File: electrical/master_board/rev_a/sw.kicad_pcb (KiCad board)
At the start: 2 copper layers, 64.7 x 45 mm, 0 parts

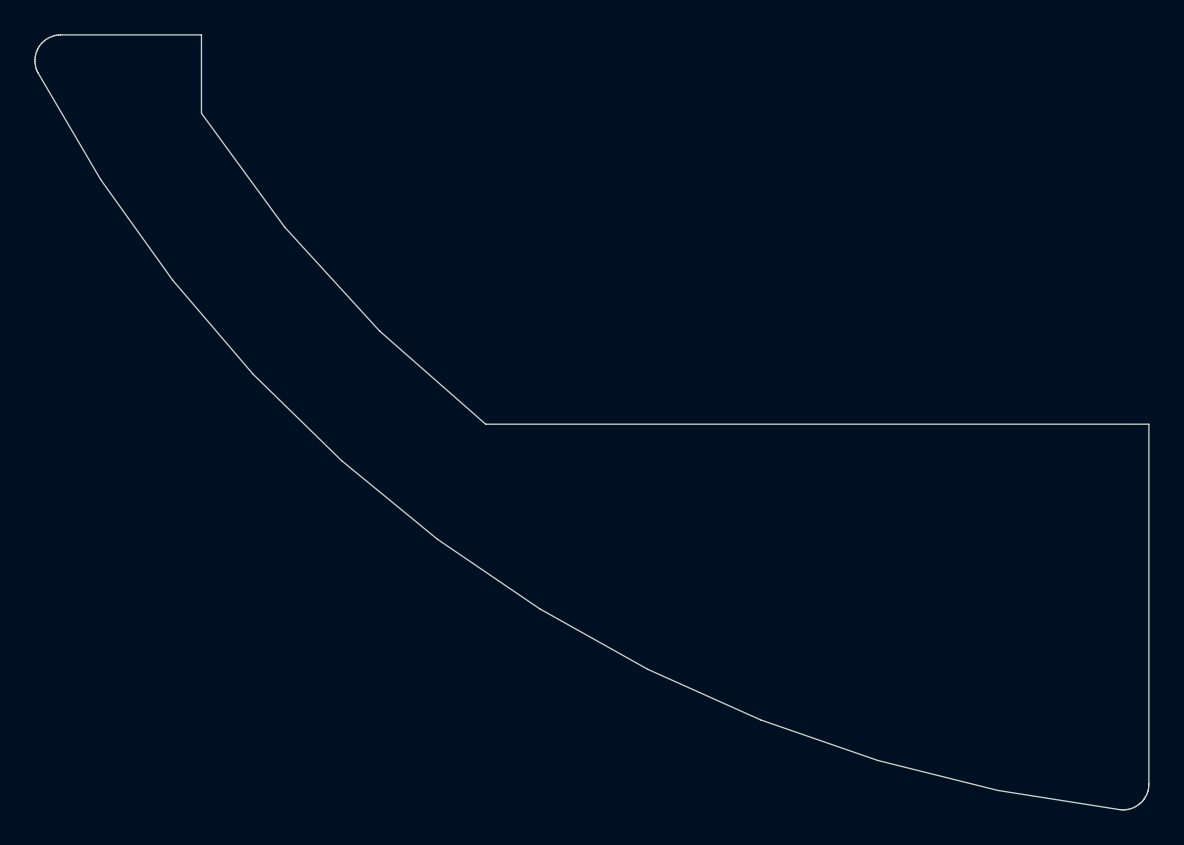
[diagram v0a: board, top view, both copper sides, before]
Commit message: Finally have everything fitting together.
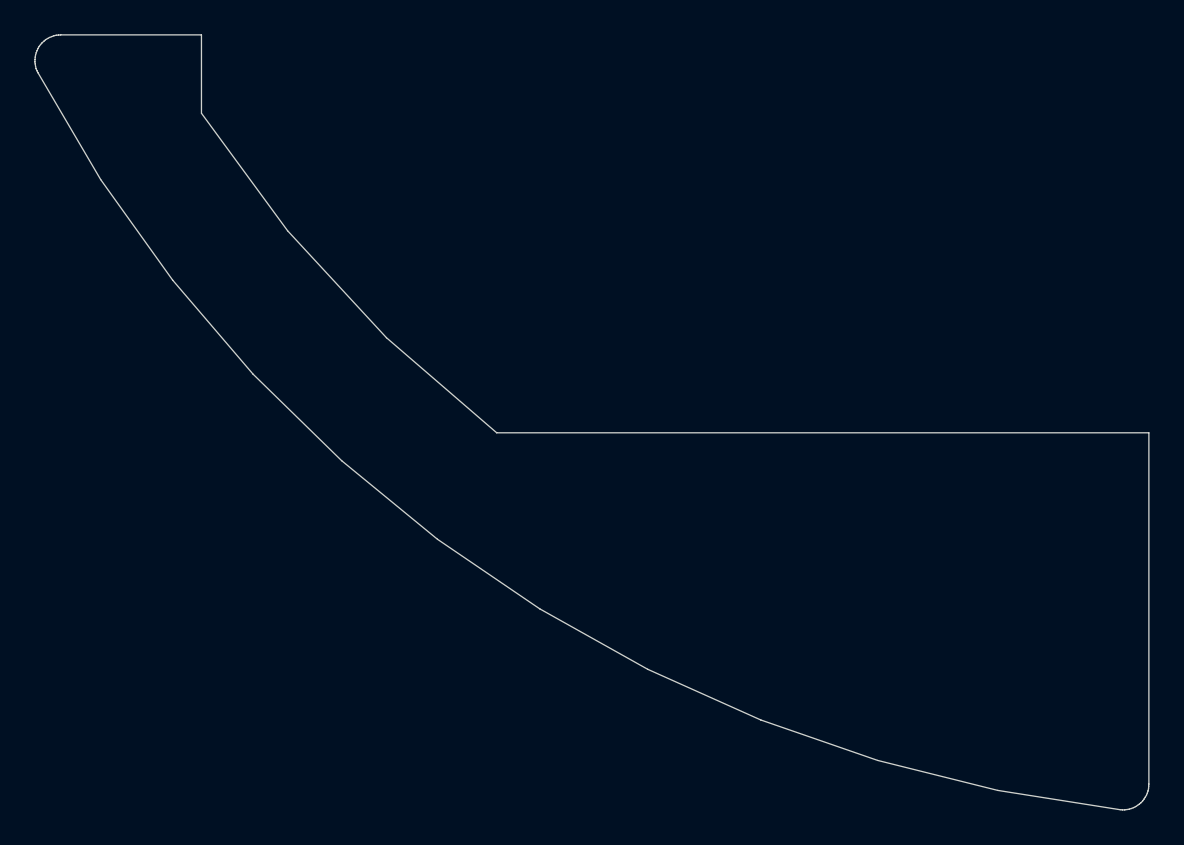
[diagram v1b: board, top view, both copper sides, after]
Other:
- outline, holes or cut-outs redrawn
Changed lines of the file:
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@@
   (gr_line (start 92.48 179.76) (end 92.49 179.62) (layer Edge.Cuts) (width 0.05))
   (gr_line (start 92.49 179.62) (end 92.5 179.49) (layer Edge.Cuts) (width 0.05))
-  (gr_line (start 92.5 179.49) (end 92.5 158.6) (layer Edge.Cuts) (width 0.05))
-  (gr_line (start 92.5 158.6) (end 54 158.6) (layer Edge.Cuts) (width 0.05))
-  (gr_line (start 54 158.6) (end 47.85 153.2) (layer Edge.Cuts) (width 0.05))
-  (gr_line (start 47.85 153.2) (end 42.33 147.16) (layer Edge.Cuts) (width 0.05))
-  (gr_line (start 42.33 147.16) (end 37.5 140.55) (layer Edge.Cuts) (width 0.05))
+  (gr_line (start 92.5 179.49) (end 92.5 159.1) (layer Edge.Cuts) (width 0.05))
+  (gr_line (start 92.5 159.1) (end 54.64 159.1) (layer Edge.Cuts) (width 0.05))
+  (gr_line (start 54.64 159.1) (end 48.24 153.58) (layer Edge.Cuts) (width 0.05))
+  (gr_line (start 48.24 153.58) (end 42.5 147.37) (layer Edge.Cuts) (width 0.05))
+  (gr_line (start 42.5 147.37) (end 37.5 140.55) (layer Edge.Cuts) (width 0.05))
   (gr_line (start 37.5 140.55) (end 37.5 136) (layer Edge.Cuts) (width 0.05))
 )
